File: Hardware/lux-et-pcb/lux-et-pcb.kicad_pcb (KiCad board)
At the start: 2 copper layers, 80 x 54 mm, 87 parts, among them J1 Conn_01x03_Socket, J2 Conn_01x03_Socket, J3 Conn_01x03_Socket, J4 USB_C_Receptacle_PowerOnly_6P, Q1 PMOS, Q2 PMOS, Q3 AO3400A, Q4 AO3400A, Q5 AO3400A, Q7 2N7002K, U1 XL1509-5V, U2 AP2112K-3.3, U3 ESP32-WROOM-32, U4 TP4056

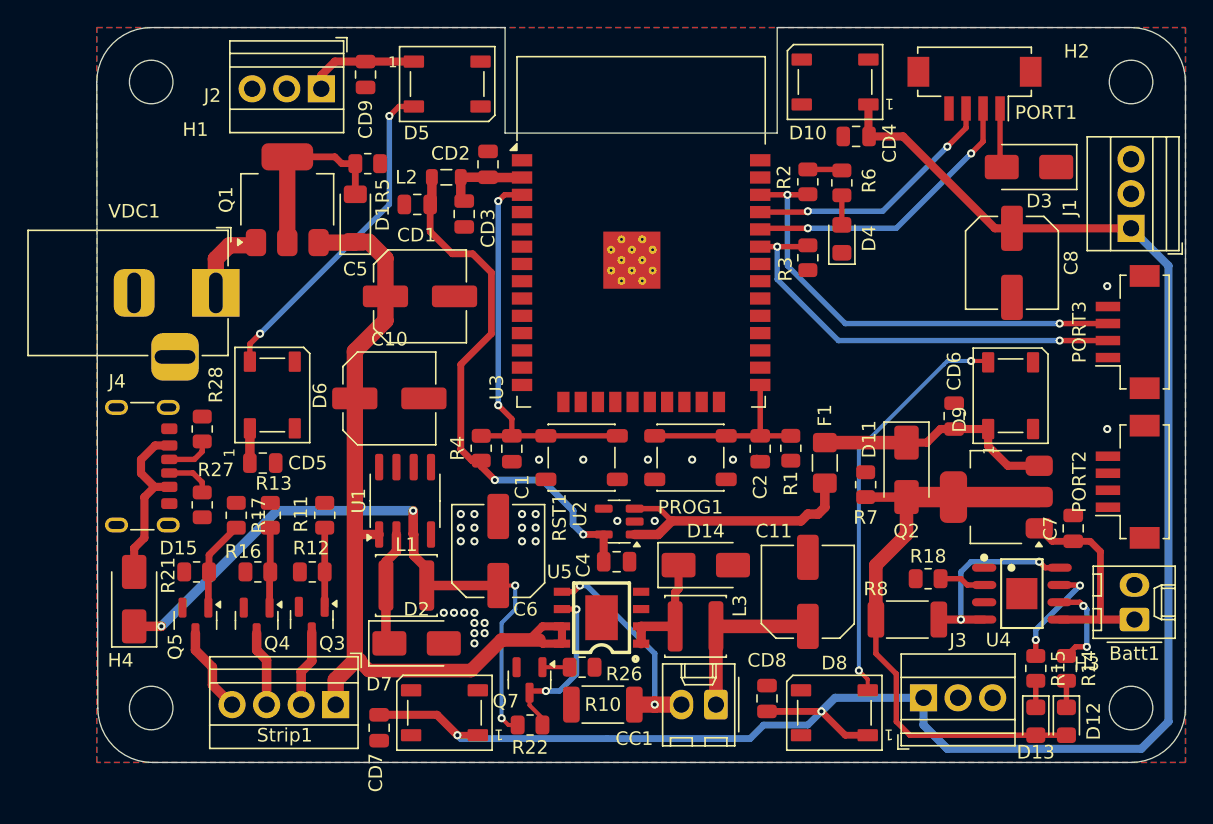
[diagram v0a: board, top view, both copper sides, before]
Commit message: First finished layout for review
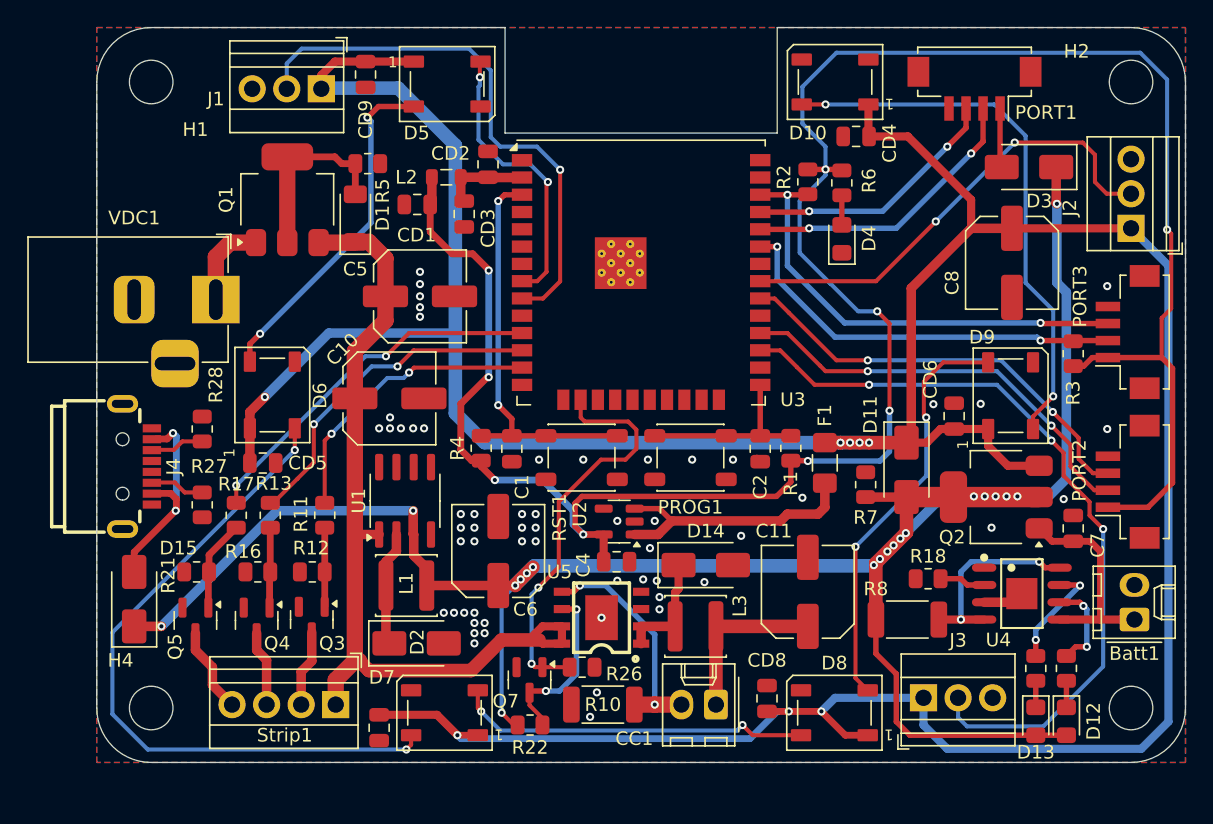
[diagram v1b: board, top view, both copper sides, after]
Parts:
- J4: footprint Connector_USB:USB_C_Receptacle_GCT_USB4125-xx-x-0190_6P_TopMnt_Horizontal -> Library:USB-C-SMD_GT-USB-7101A
- U3: footprint RF_Module:ESP32-WROOM-32 -> RF_Module:ESP32-WROOM-32U
- moved J1 60.4 mm to (136.2, 57.2), turned to 180 degrees
- moved J2 60.4 mm to (195.8, 67.5), turned to 90 degrees
- moved R3 20.7 mm to (191.5, 76.7)
- moved J4 0.72 mm to (122.7, 85.0)
- moved VDC1 0.49 mm to (128.5, 72.7)
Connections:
- PORT2 pad 2: IO2 -> IO17
- PORT2 pad 3: IO4 -> IO18
- U3 pad 11: unconnected-(U3-IO26-Pad11) -> CH3
- U3 pad 12: unconnected-(U3-IO27-Pad12) -> CH2
- U3 pad 13: unconnected-(U3-IO14-Pad13) -> CH1
- U3 pad 16: unconnected-(U3-IO13-Pad16) -> CH0
- U3 pad 24: IO2 -> unconnected-(U3-IO2-Pad24)
- U3 pad 26: IO4 -> unconnected-(U3-IO4-Pad26)
- U3 pad 27: unconnected-(U3-IO16-Pad27) -> WLED_3
- U3 pad 28: unconnected-(U3-IO17-Pad28) -> IO17
- U3 pad 30: unconnected-(U3-IO18-Pad30) -> IO18
- U3 pad 31: unconnected-(U3-IO19-Pad31) -> WLED_2
- U3 pad 8: unconnected-(U3-IO32-Pad8) -> WLED_0
- U3 pad 9: unconnected-(U3-IO33-Pad9) -> WLED_1
- U5 pad 4: Net-(U5-FB) -> GND
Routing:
- net +3.3V: track 41.9 -> 173.1 mm, vias 2 -> 9
- net V_REG: track 163.7 -> 263.3 mm, vias 2 -> 8
- net +5V: track 91.7 -> 158.8 mm, vias 4 -> 19
- net WLED_3: track 0.00 -> 56.6 mm, vias 0 -> 3
- net Net-(D6-DOUT): track 0.00 -> 50.4 mm, vias 0 -> 2
- net WLED_1: track 0.00 -> 40.5 mm, vias 0 -> 1
- net Net-(D10-DIN): track 0.00 -> 40.4 mm, vias 0 -> 2
- net WLED_2: track 0.00 -> 34.2 mm, vias 0 -> 2
- net IO18: track 0.00 -> 31.8 mm, vias 0 -> 2
- net IO17: track 0.00 -> 31.3 mm, vias 0 -> 2
- net CH0: track 2.00 -> 30.0 mm, vias 0 -> 2
- net CH3: track 0.00 -> 26.9 mm, vias 0 -> 2
- net Net-(D7-DOUT): track 0.00 -> 26.2 mm, vias 0 -> 2
- net CH2: track 0.00 -> 24.8 mm, vias 0 -> 2
- net CH1: track 0.00 -> 21.3 mm, vias 0 -> 2
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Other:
- outline, holes or cut-outs redrawn
